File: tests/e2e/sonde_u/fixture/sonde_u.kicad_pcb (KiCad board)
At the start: 2 copper layers, 80.4 x 43.2 mm, 25 parts, among them J1 DB25MALE, J2 DB9MALE, P1 CONN_6, U1 74LS125, U2 74LS125

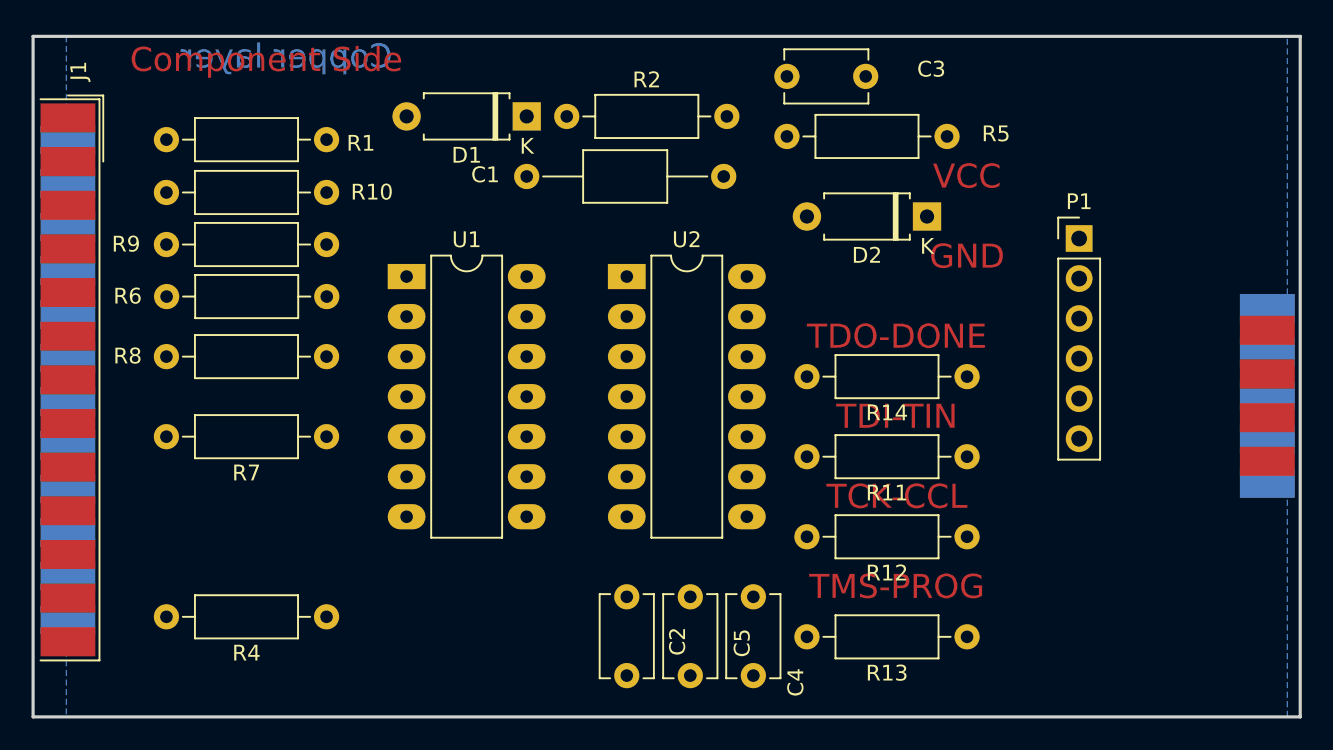
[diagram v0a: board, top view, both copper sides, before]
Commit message: e2e
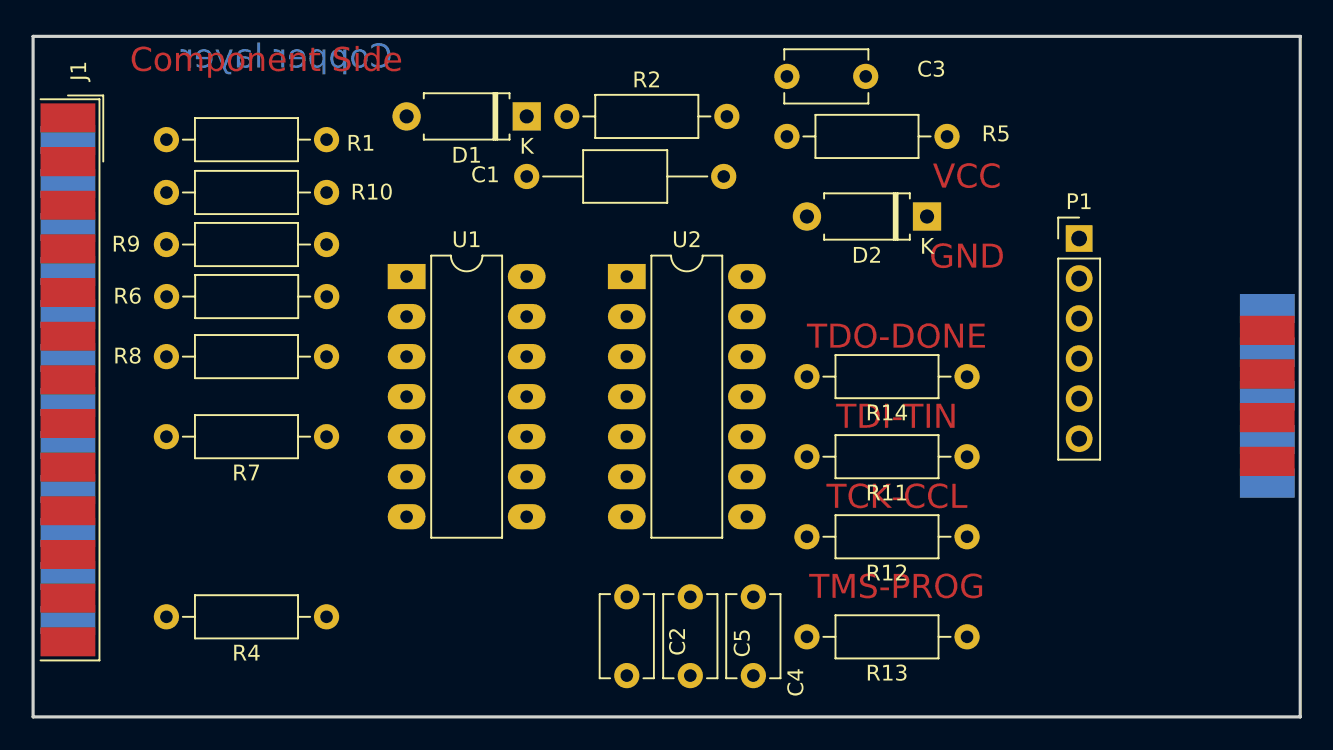
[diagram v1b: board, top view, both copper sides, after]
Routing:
- removed copper zone on B.Cu, net GND
